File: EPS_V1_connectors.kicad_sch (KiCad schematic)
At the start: 11 parts, among them J1 Conn_01x20, J2 Conn_01x30, J3 Conn_01x15, J4 Conn_01x04, SW1 SWITCH, SW2 SWITCH, SW3 SWITCH

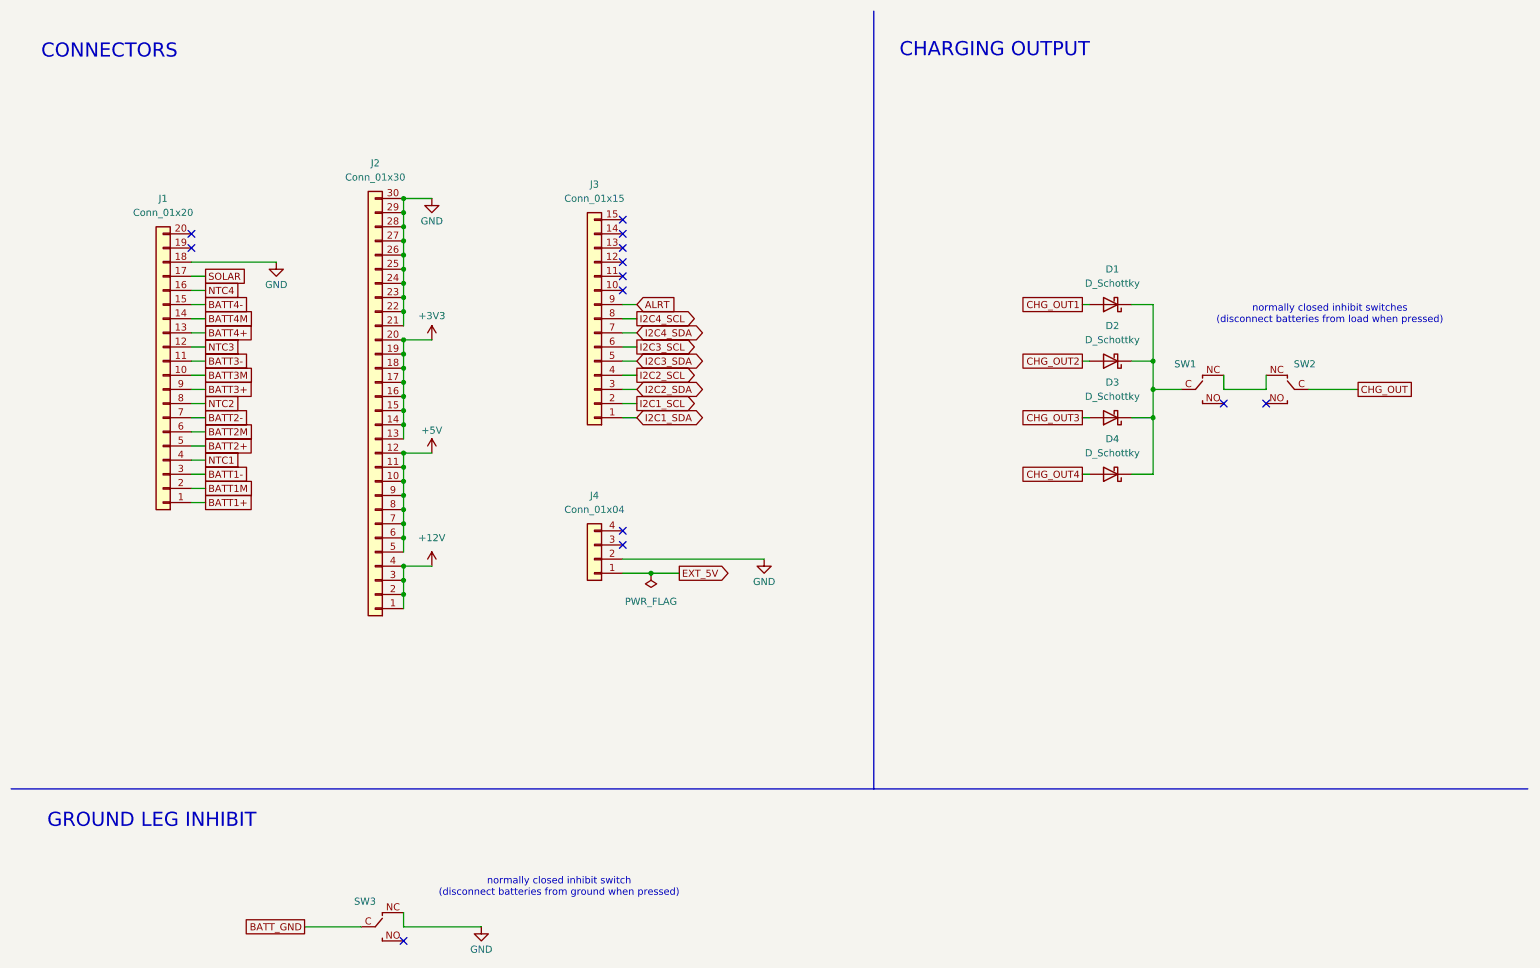
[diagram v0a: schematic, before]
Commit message: Do layout draft
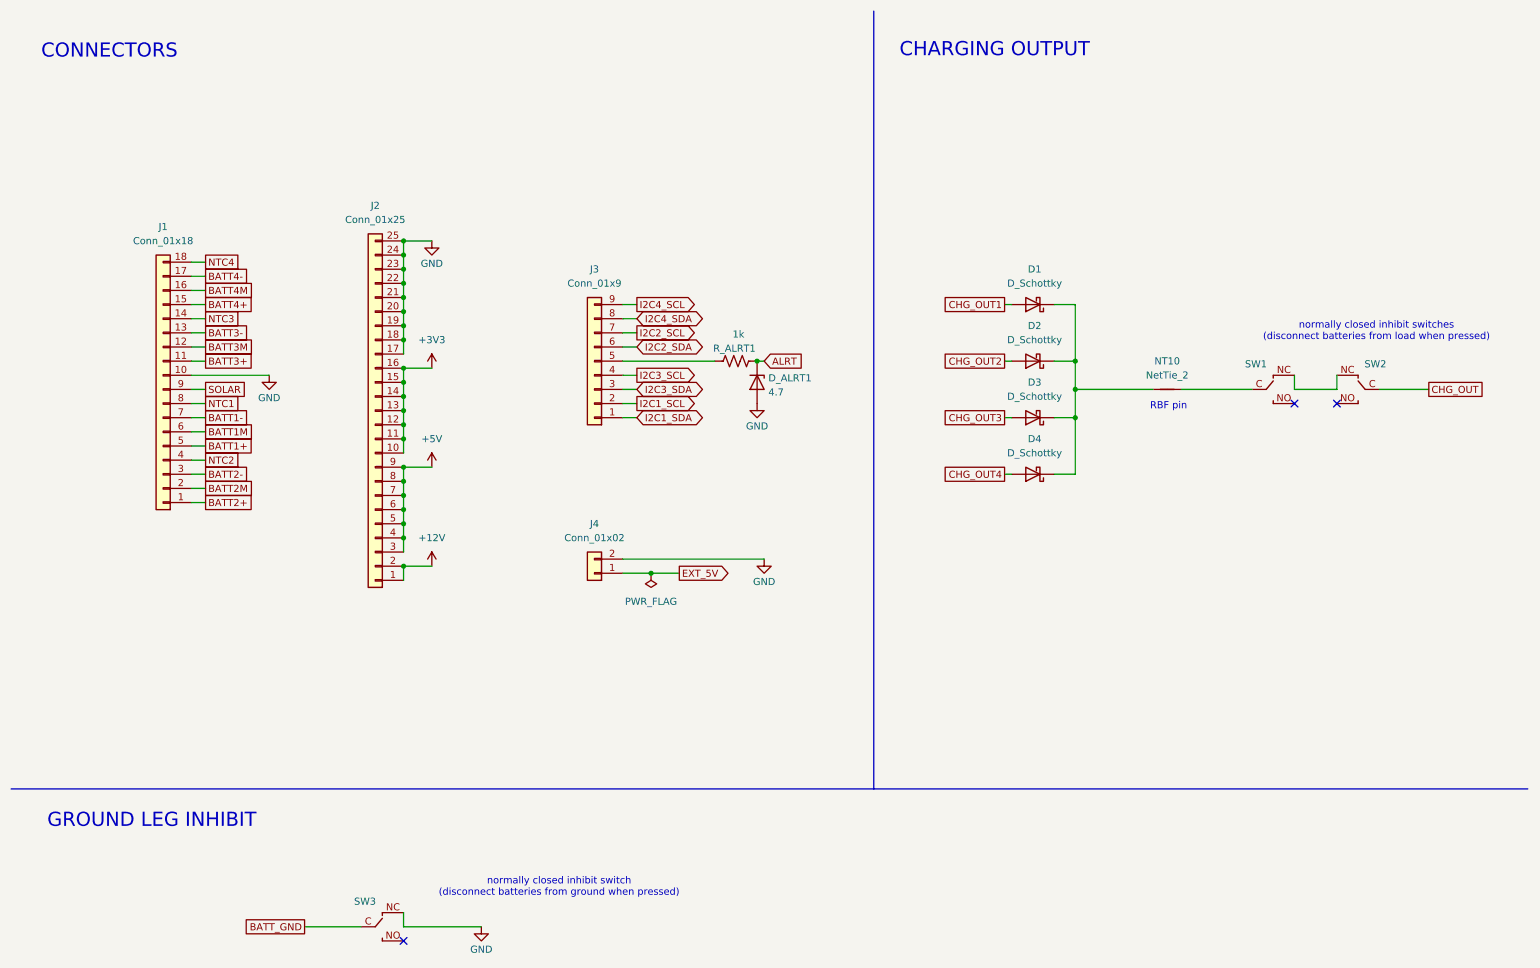
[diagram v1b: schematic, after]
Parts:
- removed J1: Conn_01x20, Connector_IDC:IDC-Header_2x10_P2.54mm_Latch6.5mm_Vertical, symbol Connector_Generic:Conn_01x20
- removed J2: Conn_01x30, Connector_PinHeader_2.54mm:PinHeader_1x30_P2.54mm_Vertical, symbol Connector_Generic:Conn_01x30
- removed J3: Conn_01x15, Connector_PinHeader_2.54mm:PinHeader_1x15_P2.54mm_Vertical, symbol Connector_Generic:Conn_01x15
- removed J4: Conn_01x04, Connector_PinHeader_2.54mm:PinHeader_1x04_P2.54mm_Vertical, symbol Connector_Generic:Conn_01x04
- added D_ALRT1: 4.7, Diode_SMD:D_0603_1608Metric, symbol Device:D_Zener
- added J1: Conn_01x18, Connector_PinHeader_2.54mm:PinHeader_1x18_P2.54mm_Vertical, symbol Connector_Generic:Conn_01x18
- added J2: Conn_01x25, Connector_PinHeader_2.54mm:PinHeader_1x25_P2.54mm_Vertical, symbol Connector_Generic:Conn_01x25
- added J3: Conn_01x9, Connector_PinHeader_2.54mm:PinHeader_1x09_P2.54mm_Vertical, symbol Connector_Generic:Conn_01x09
- added J4: Conn_01x02, Connector_PinHeader_2.54mm:PinHeader_1x02_P2.54mm_Vertical, symbol Connector_Generic:Conn_01x02
- added NT10: NetTie_2, switches:RBF, symbol Device:NetTie_2
- added R_ALRT1: 1k, Resistor_SMD:R_0603_1608Metric, symbol Device:R_US
- SW1, SW3: footprint switches:D2F-L3-D-HORIZONTAL-R -> switches:SWITCH-R
- SW2: footprint switches:D2F-L3-D-HORIZONTAL-L -> switches:SWITCH-L
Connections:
- net ALRT: now also D_ALRT1.1 (K), R_ALRT1.1
- net BATT1+: now also J1.5 (Pin_5)
- net BATT1-: now also J1.7 (Pin_7)
- net BATT1M: now also J1.6 (Pin_6)
- net BATT2+: now also J1.1 (Pin_1)
- net BATT2-: now also J1.3 (Pin_3)
- net BATT2M: now also J1.2 (Pin_2)
- net BATT3+: now also J1.11 (Pin_11)
- net BATT3-: now also J1.13 (Pin_13)
- net BATT3M: now also J1.12 (Pin_12)
- net BATT4+: now also J1.15 (Pin_15)
- net BATT4-: now also J1.17 (Pin_17)
- net BATT4M: now also J1.16 (Pin_16)
- net EXT_5V: now also J4.1 (Pin_1)
- net GND: now also D_ALRT1.2 (A), J1.10 (Pin_10), J2.17 (Pin_17), J2.18 (Pin_18), J2.19 (Pin_19), J2.20 (Pin_20), J2.21 (Pin_21), J2.22 (Pin_22), J2.23 (Pin_23), J2.24 (Pin_24), J2.25 (Pin_25), J4.2 (Pin_2)
- net I2C1_SCL: now also J3.2 (Pin_2)
- net I2C1_SDA: now also J3.1 (Pin_1)
- net I2C2_SCL: now also J3.7 (Pin_7)
- net I2C2_SDA: now also J3.6 (Pin_6)
- net I2C3_SCL: now also J3.4 (Pin_4)
- net I2C3_SDA: now also J3.3 (Pin_3)
- net I2C4_SCL: now also J3.9 (Pin_9)
- net I2C4_SDA: now also J3.8 (Pin_8)
- net NTC1: now also J1.8 (Pin_8)
- net NTC2: now also J1.4 (Pin_4)
- net NTC3: now also J1.14 (Pin_14)
- net NTC4: now also J1.18 (Pin_18)
- net SOLAR: now also J1.9 (Pin_9)
- net at D1.1 (K), D2.1 (K), D3.1 (K)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: now also NT10.1; no longer SW1.C (COM)
- new net: NT10.2, SW1.C (COM)
- new net: J3.5 (Pin_5), R_ALRT1.2
- new net +12V: J2.1 (Pin_1), J2.2 (Pin_2)
- new net +3V3: J2.10 (Pin_10), J2.11 (Pin_11), J2.12 (Pin_12), J2.13 (Pin_13), J2.14 (Pin_14), J2.15 (Pin_15), J2.16 (Pin_16)
- new net +5V: J2.3 (Pin_3), J2.4 (Pin_4), J2.5 (Pin_5), J2.6 (Pin_6), J2.7 (Pin_7), J2.8 (Pin_8), J2.9 (Pin_9)
- no-connect marks 13 -> 3
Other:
- note added: "RBF pin"
- moved on the sheet: D1, D2, D3, D4, SW1, SW2
